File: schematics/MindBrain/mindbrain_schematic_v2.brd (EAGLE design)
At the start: 81 x 47.6 mm, 51 parts, among them CON1 POWER, IC1 TL084, IC2 TL084

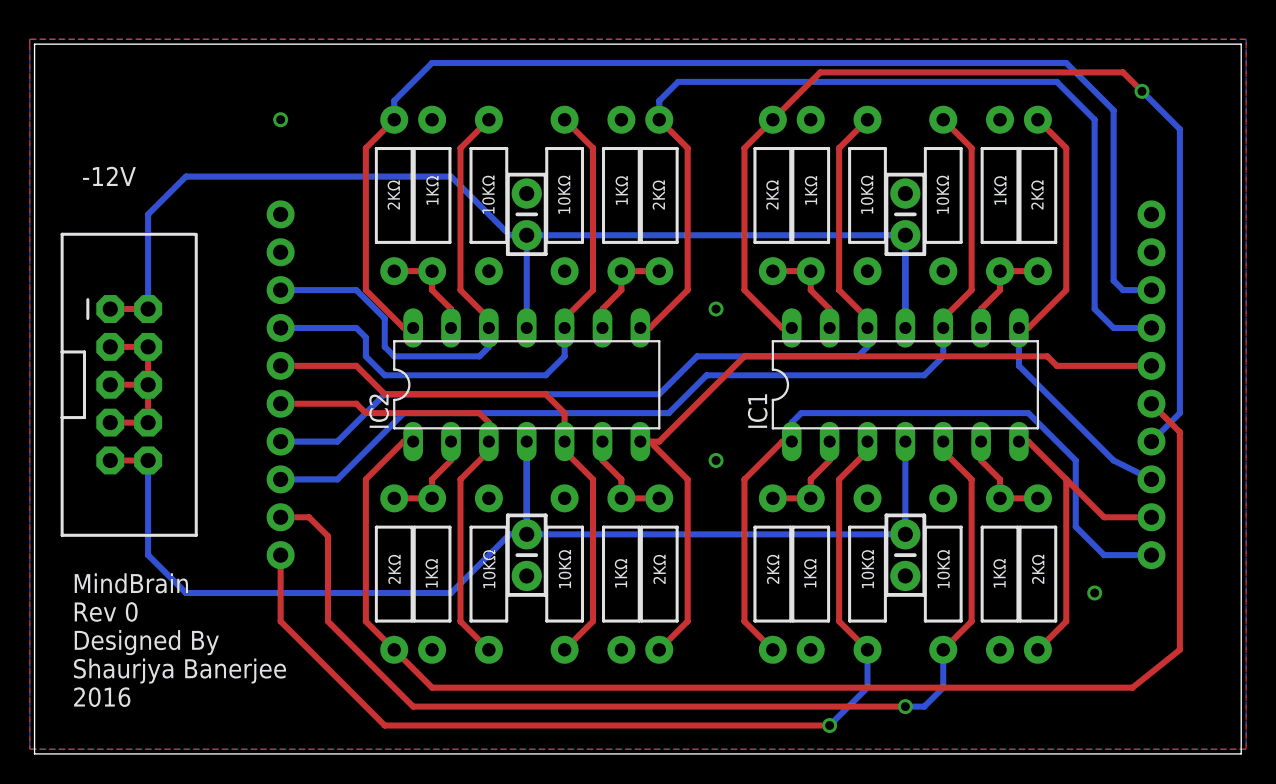
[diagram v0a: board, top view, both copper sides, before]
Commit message: getting ERC warnings, not sure why?
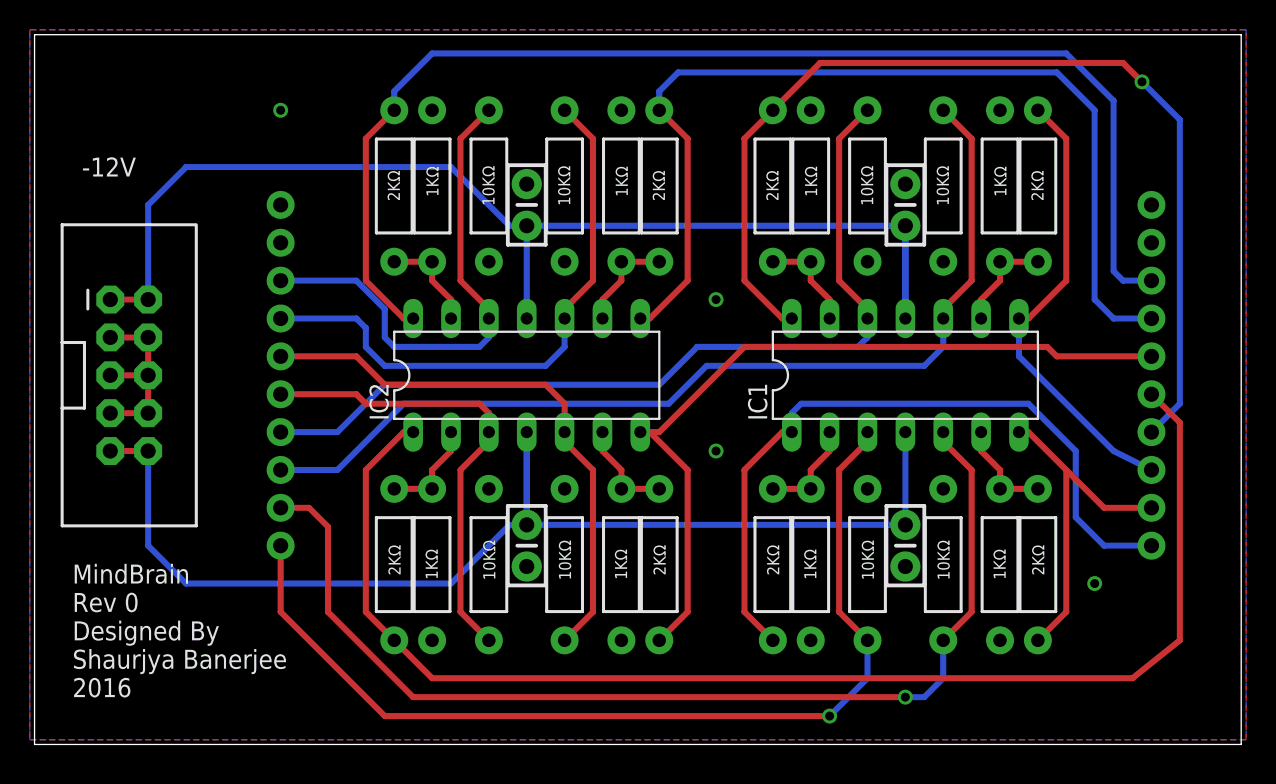
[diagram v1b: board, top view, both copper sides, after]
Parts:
- moved R3 0.64 mm to (64.8, 37.5)
- moved R4 0.64 mm to (52.1, 37.5)
- moved R7 0.64 mm to (39.4, 37.5)
- moved R8 0.64 mm to (26.7, 37.5)
- moved RF3 0.64 mm to (67.3, 37.5)
- moved RF4 0.64 mm to (49.5, 37.5)
- moved RF7 0.64 mm to (41.9, 37.5)
- moved RF8 0.64 mm to (24.1, 37.5)
- moved RIN3 0.64 mm to (61.0, 37.5)
- moved RIN4 0.64 mm to (55.9, 37.5)
- moved RIN7 0.64 mm to (35.6, 37.5)
- moved RIN8 0.64 mm to (30.5, 37.5)
- moved C1 0.64 mm to (33.0, 13.3)
- moved C3 0.64 mm to (58.4, 13.3)
- moved CON1 0.64 mm to (6.35, 24.8)
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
